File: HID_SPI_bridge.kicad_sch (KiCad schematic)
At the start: 10 parts, among them P1 USB_C_Plug_USB2.0, U1 STM32F042K4Tx

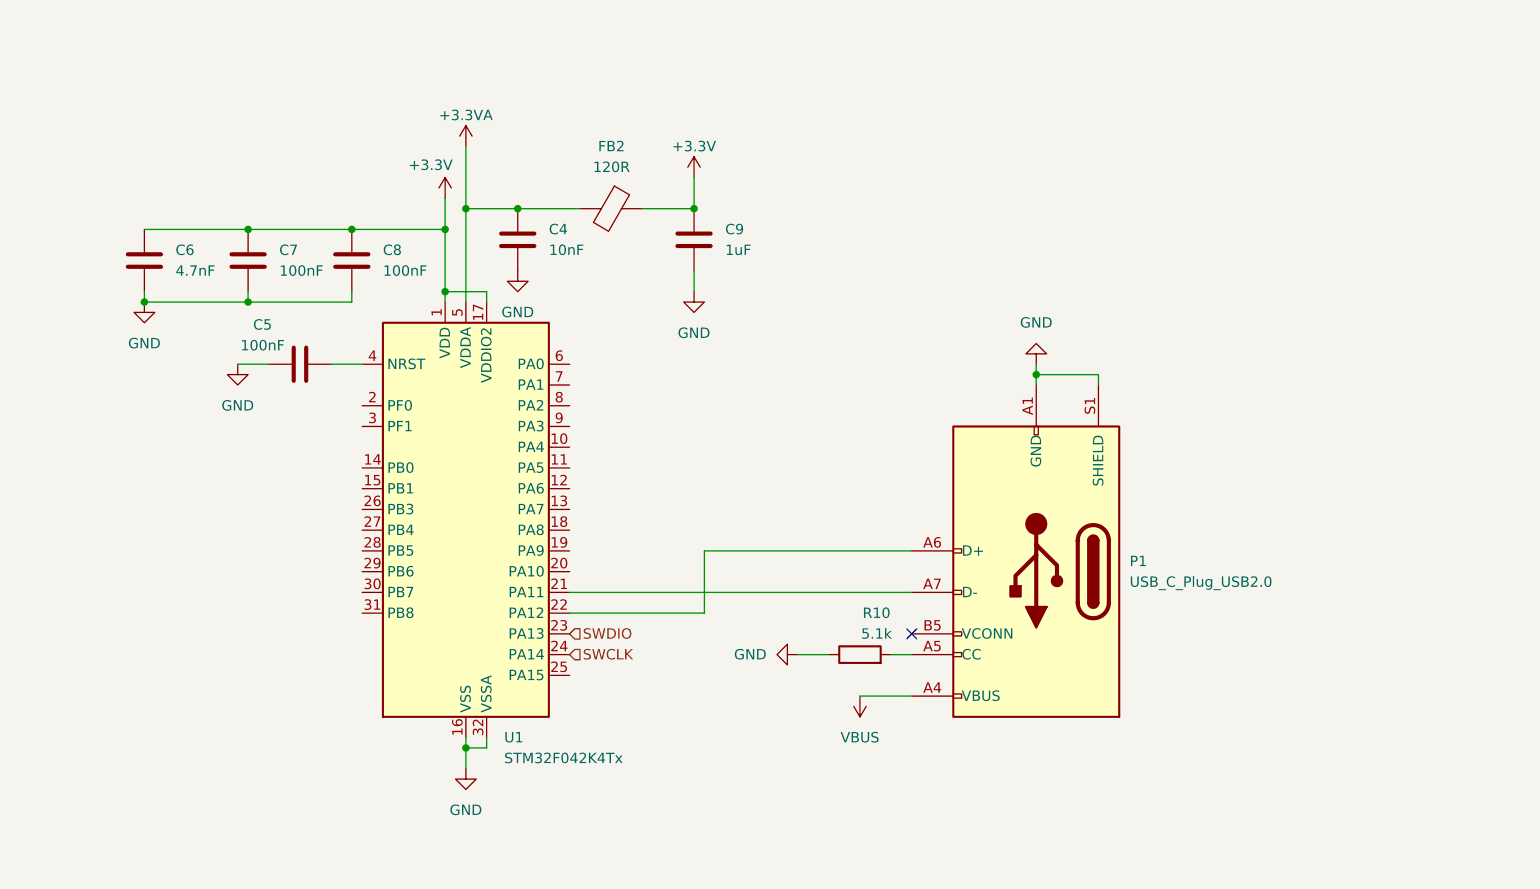
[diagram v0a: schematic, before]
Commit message: [ADD](General) v1
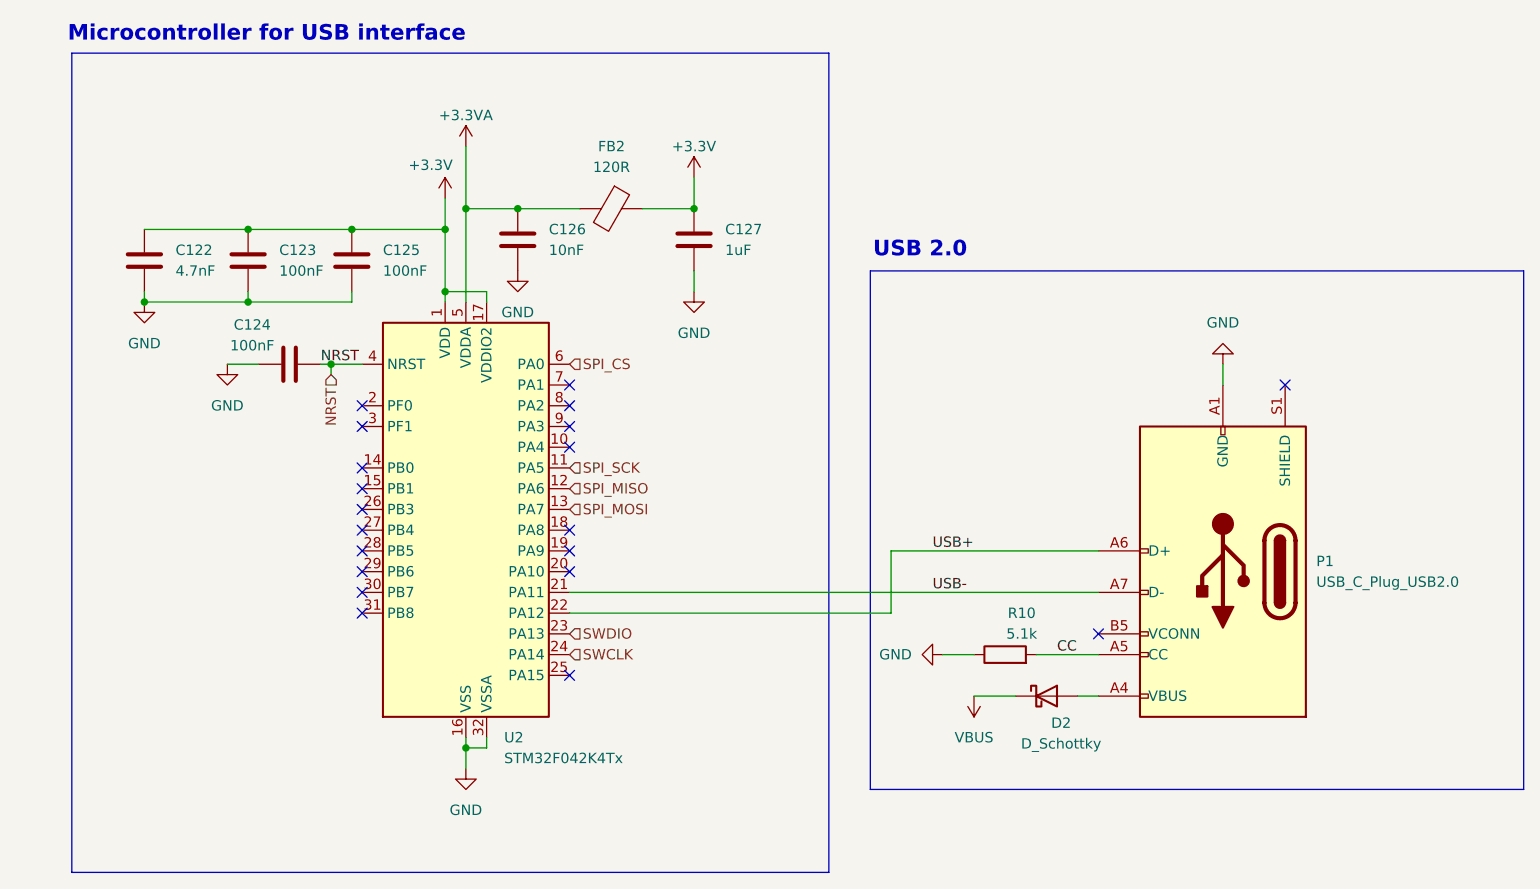
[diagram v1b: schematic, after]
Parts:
- added D2: D_Schottky, symbol Device:D_Schottky
- renumbered C6 to C122, C7 to C123, C5 to C124, C8 to C125, C4 to C126, C9 to C127, U1 to U2
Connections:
- net GND: no longer P1.S1 (SHIELD)
- net VBUS: now also D2.1 (K); no longer P1.A4 (VBUS), P1.A9 (VBUS), P1.B4 (VBUS), P1.B9 (VBUS)
- net NRST: now reaches C124.2, U2.4 (NRST)
- net CC: now reaches P1.A5 (CC), R10.2
- net SPI_SCK: now reaches U2.11 (PA5)
- net SPI_MISO: now reaches U2.12 (PA6)
- net SPI_MOSI: now reaches U2.13 (PA7)
- net USB-: now reaches P1.A7 (D-), U2.21 (PA11)
- net USB+: now reaches P1.A6 (D+), U2.22 (PA12)
- net SPI_CS: now reaches U2.6 (PA0)
- new net: D2.2 (A), P1.A4 (VBUS), P1.A9 (VBUS), P1.B4 (VBUS), P1.B9 (VBUS)
- no-connect marks 1 -> 20
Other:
- note added: "Microcontroller for USB interface"
- note added: "USB 2.0"
- company: (none) -> Ryzzen
- title: (none) -> TMR based triple USB Keyboard
- moved on the sheet: C124, P1, R10
